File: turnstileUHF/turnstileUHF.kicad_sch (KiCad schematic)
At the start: 54 parts, among them J5 RFPC-SMA28-F, Q1 2N7002, Q2 2N7002, Q3 2N7002, Q4 2N7002, Q5 AO3401A, Q6 AO3401A, Q7 AO3401A, Q8 2N7002, U1 74HCT238D

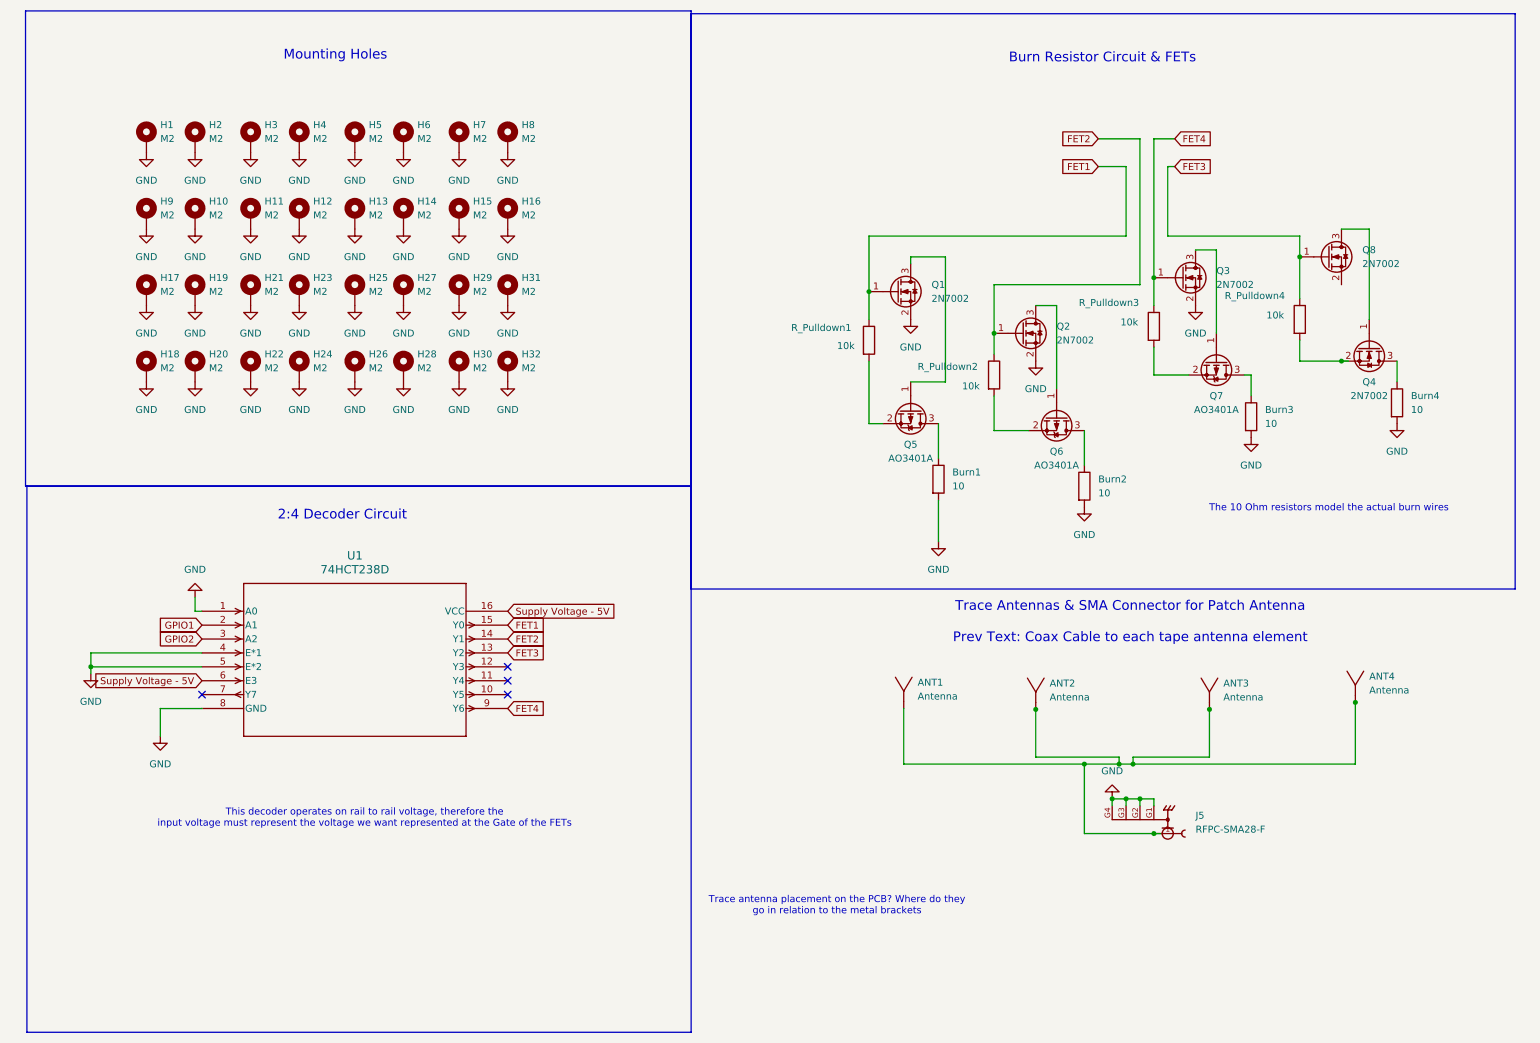
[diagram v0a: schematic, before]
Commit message: door sensing not update?
tryint to push changes
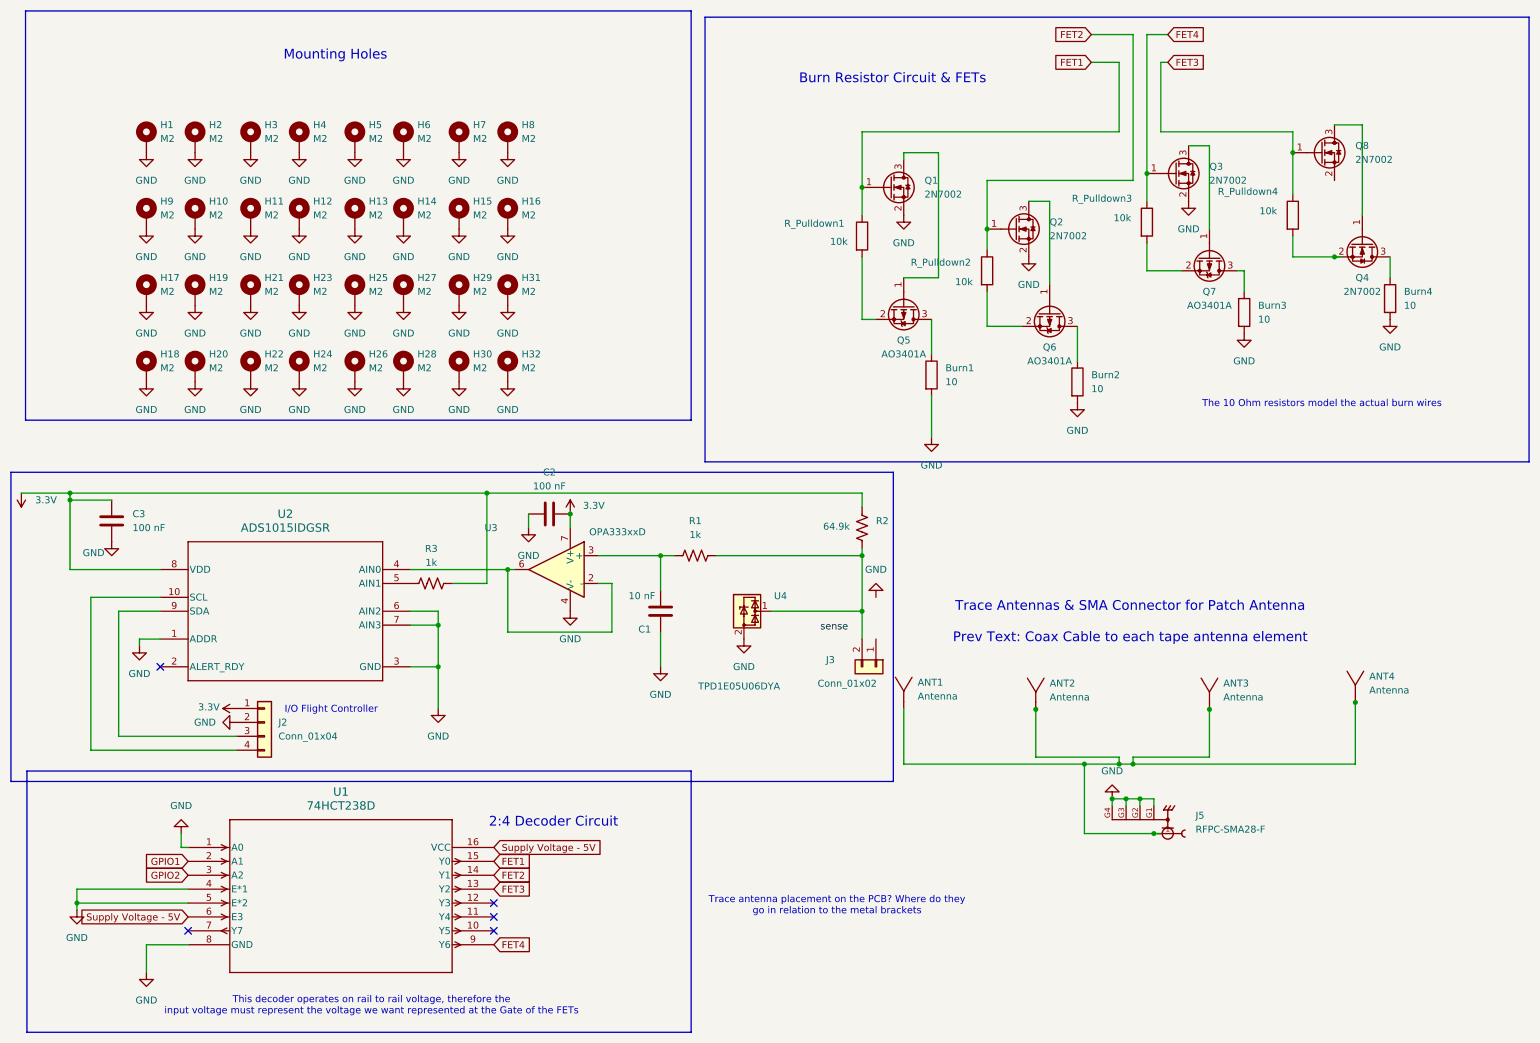
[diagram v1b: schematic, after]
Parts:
- added C1: 10 nF, Capacitor_SMD:C_0603_1608Metric, symbol Device:C
- added C2, C3: 100 nF, Capacitor_SMD:C_0603_1608Metric, symbol Device:C
- added J2: Conn_01x04, Connector_JST:JST_PH_S4B-PH-K_1x04_P2.00mm_Horizontal, symbol Connector_Generic:Conn_01x04
- added J3: Conn_01x02, Connector_JST:JST_PH_S2B-PH-K_1x02_P2.00mm_Horizontal, symbol Connector_Generic:Conn_01x02
- added R1, R3: 1k, Resistor_SMD:R_0603_1608Metric, symbol Device:R_US
- added R2: 64.9k, Resistor_SMD:R_0603_1608Metric, symbol Device:R_US
- added U2: ADS1015IDGSR, ADS1115:DGS0010A_M, symbol ADS1115:ADS1115IDGSR
- added U3: OPA333xxD, Package_SO:SOIC-8_3.9x4.9mm_P1.27mm, symbol Amplifier_Operational:OPA333xxD
- added U4: TPD1E05U06DYA, Diode_SMD:D_SOD-523, symbol Power_Protection:TPD1E05U06DYA
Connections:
- net GND: now also C1.2, C2.1, C3.2, J2.2 (Pin_2), U2.1 (ADDR), U2.3 (GND), U2.6 (AIN2), U2.7 (AIN3), U3.4 (V-), U4.2 (GND)
- new net: J3.2 (Pin_2), R1.1, R2.2, U4.1 (I/O)
- new net: C1.1, R1.2, U3.3 (+)
- new net: U2.4 (AIN0), U3.2 (-), U3.6
- new net: J2.4 (Pin_4), U2.10 (SCL)
- new net: R3.1, U2.5 (AIN1)
- new net: J2.3 (Pin_3), U2.9 (SDA)
- new net 3.3V: C2.2, C3.1, J2.1 (Pin_1), R2.1, R3.2, U2.8 (VDD), U3.7 (V+)
- no-connect marks 4 -> 5
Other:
- note added: "I/O Flight Controller"
- moved on the sheet: Burn1, Burn2, Burn3, Burn4, Q1, Q2, Q3, Q4, Q5, Q6, Q7, Q8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
